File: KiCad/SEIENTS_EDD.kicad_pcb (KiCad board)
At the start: 2 copper layers, 153.9 x 110 mm, 99 parts, among them IC1 A3144EUA, J1 Conn_01x02_Pin, J201 Screw_Terminal_01x04, J3 Screw_Terminal_01x05, J4 Screw_Terminal_01x02, J7 DE9_Socket, J8 DE9_Pins, M4 Motor_DC, M5 Motor_DC, M6 Motor_DC, Q201 IRLZ44N, SW10 SW_Push, SW11 SW_Push, SW12 SW_Push, SW13 SW_Push, SW14 SW_Push, SW15 SW_Push, SW8 SW_Push, SW9 SW_Push, U1 LM2596S-5, U11 MAX3232, U2 LM1117DT-3.3, U3 MCP2562-E-SN, U4 TMP102xxDRL, U5 TB6612FNG, U6 24LC256, U67 PIC24HJ64GP504-I/PT, U7 ATtiny1616-M, U8 DRV8871DDA, Y1 8 MHz

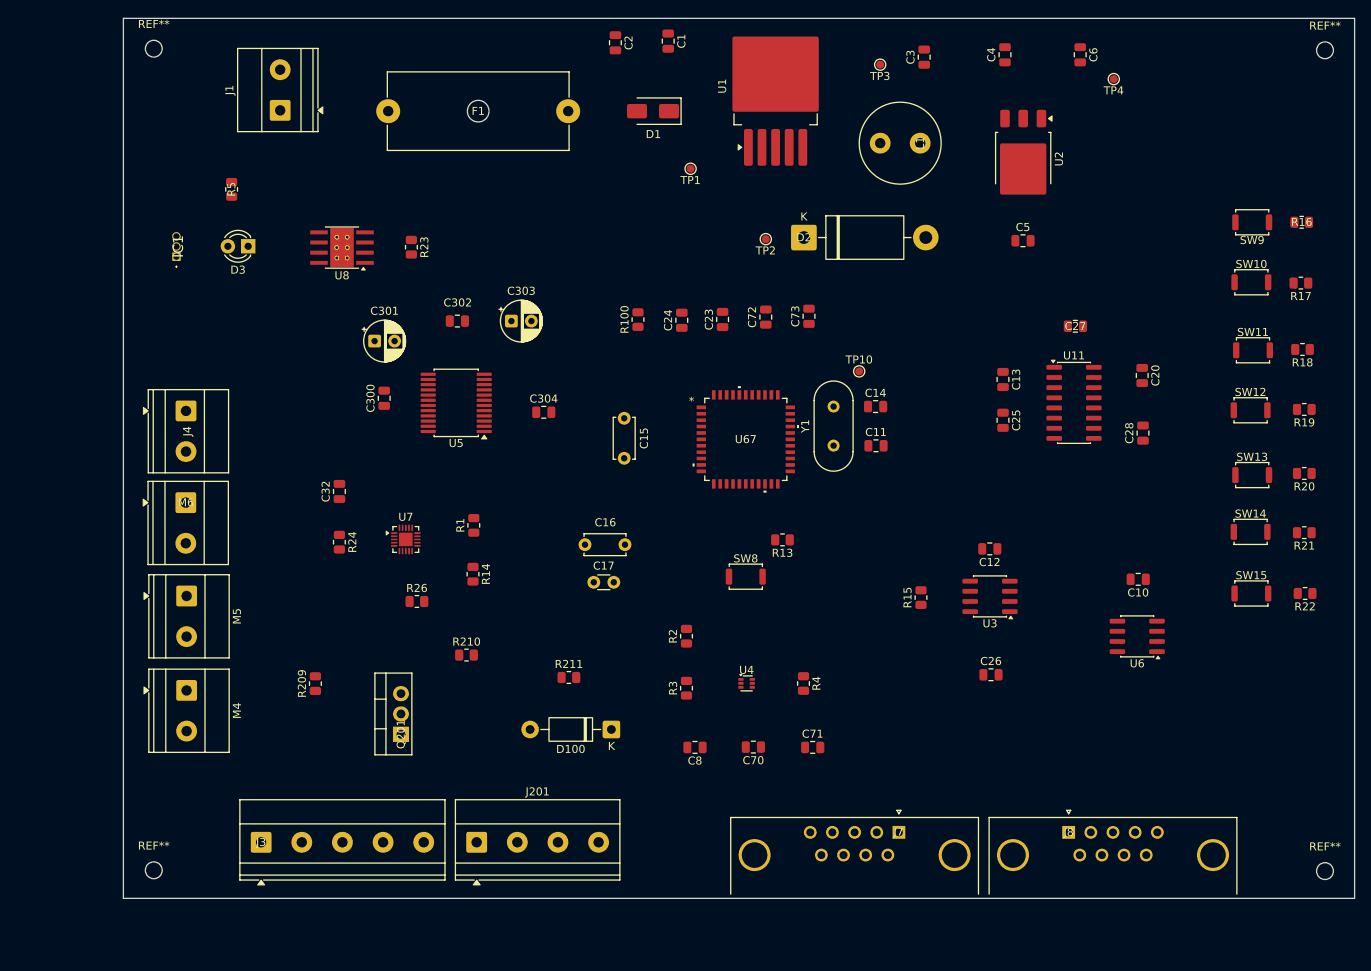
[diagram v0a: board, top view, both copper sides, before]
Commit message: cambios en el placement
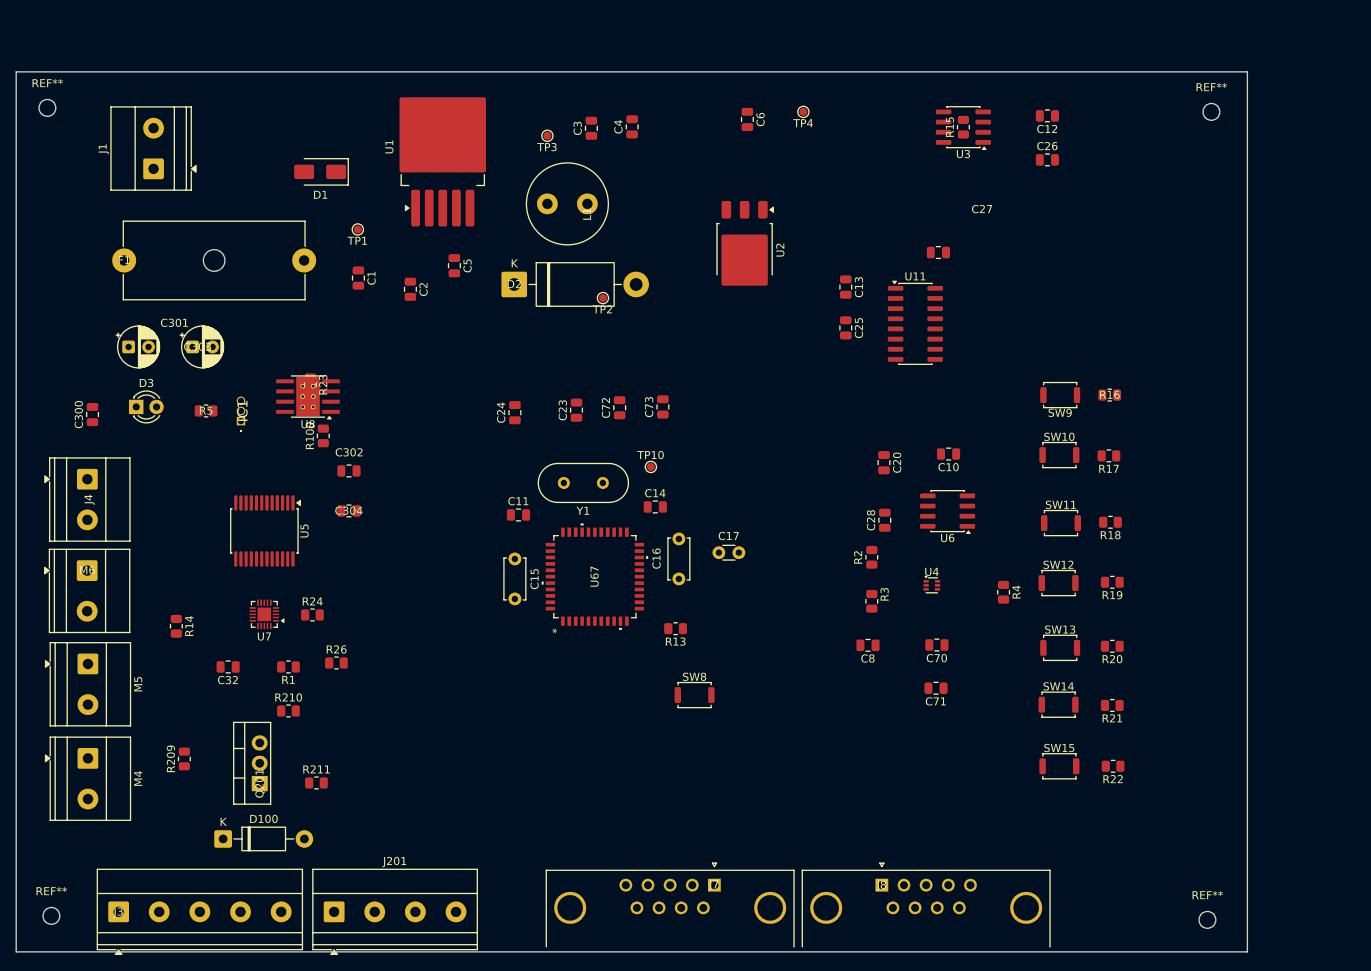
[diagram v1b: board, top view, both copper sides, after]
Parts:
- moved C5 71.1 mm to (70.9, 53.2), turned to -90 degrees
- moved C26 64.7 mm to (145.0, 40.0)
- moved R15 59.0 mm to (134.5, 35.9)
- moved U3 58.7 mm to (134.5, 35.9)
- moved C12 54.6 mm to (145.0, 34.5)
- moved D100 50.4 mm to (42.0, 124.9), turned to 0 degrees
- moved C1 48.8 mm to (58.9, 54.8)
- moved C4 47.5 mm to (93.1, 35.9)
- moved C11 45.5 mm to (78.9, 84.4)
- moved C3 42.5 mm to (88.0, 36.0)
- moved TP3 42.5 mm to (82.5, 37.0)
- moved C6 42.4 mm to (107.5, 35.0)
- moved TP1 42.3 mm to (58.8, 48.7)
- moved U1 42.3 mm to (69.4, 38.4)
- moved D1 42.3 mm to (54.1, 41.5)
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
